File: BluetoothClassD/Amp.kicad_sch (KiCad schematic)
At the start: 31 parts, among them J2 HI OUT, J3 LOW OUT, U4 TPA3110

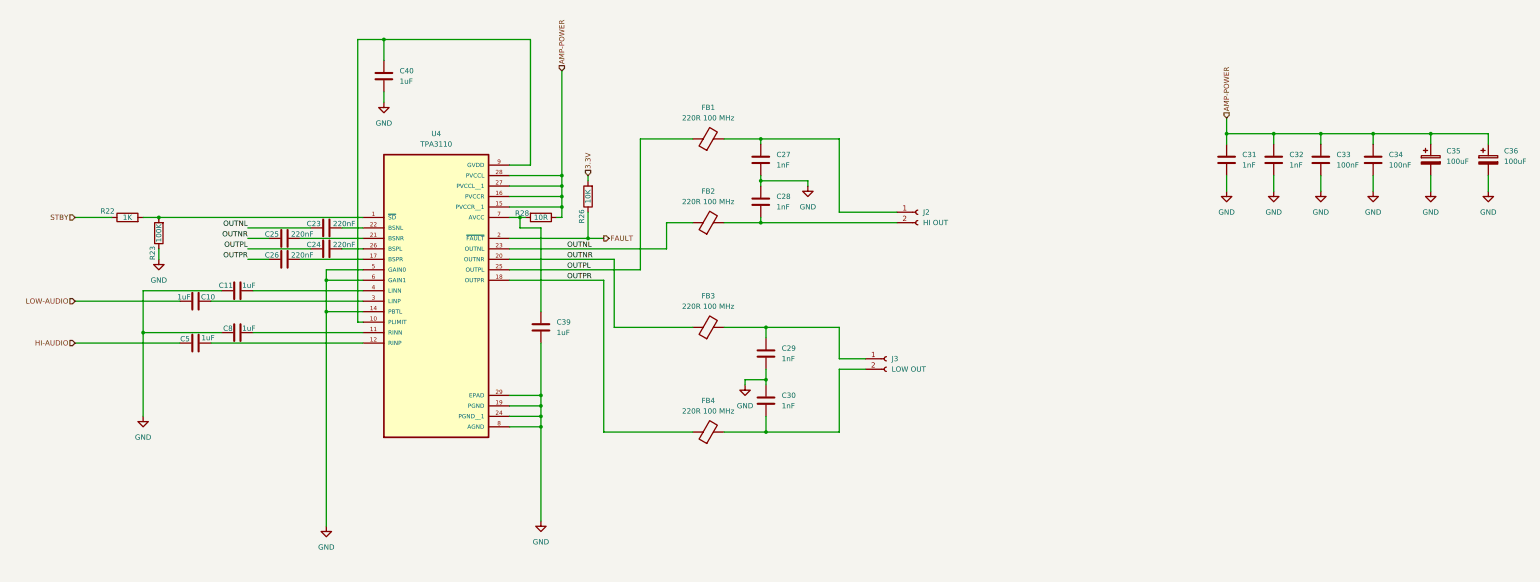
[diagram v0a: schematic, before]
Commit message: work
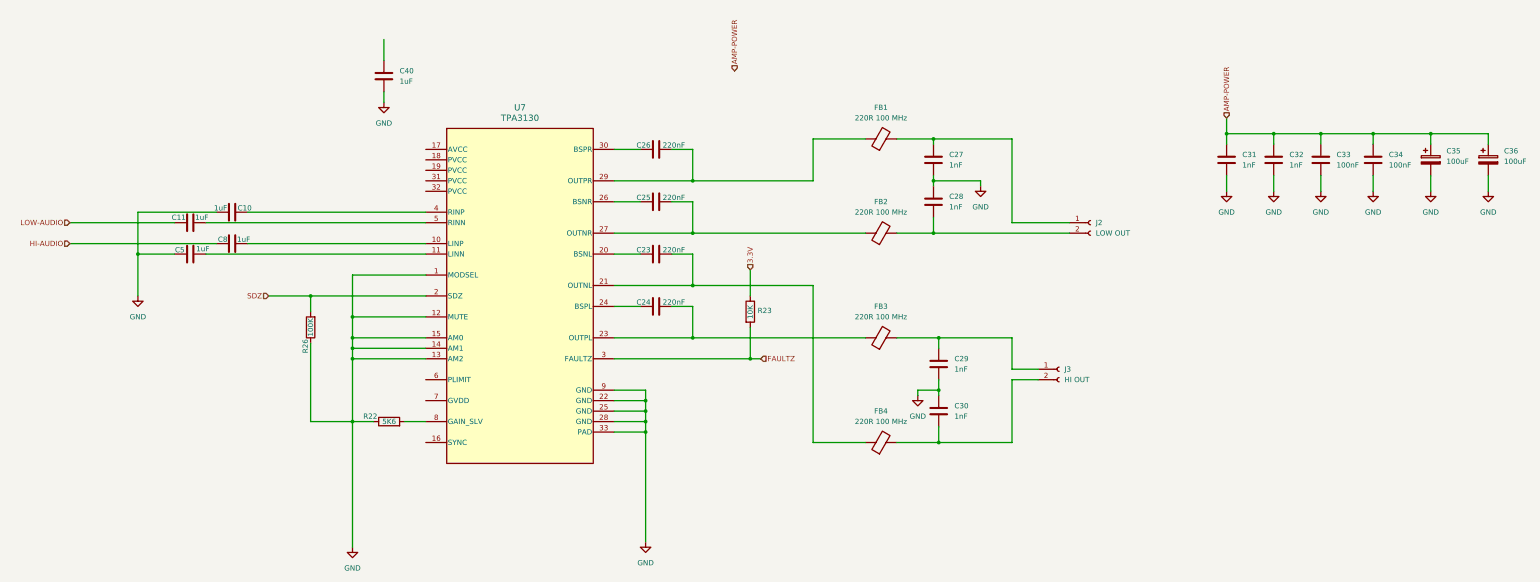
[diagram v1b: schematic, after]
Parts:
- removed C39: 1uF, Capacitor_SMD:C_1206_3216Metric_Pad1.33x1.80mm_HandSolder, symbol Device:C
- removed R28: 10R, Resistor_SMD:R_0805_2012Metric_Pad1.20x1.40mm_HandSolder, symbol Device:R
- removed U4: TPA3110, Custom:TPA3110, symbol Custom:TPA3110D2PWPR
- added U7: TPA3130, Custom:TPA3130D2DAPR, symbol Custom:TPA3130D2DAPR
- J2: value HI OUT -> LOW OUT
- J3: value LOW OUT -> HI OUT
- R22: value 1K -> 5K6
- R23: value 100K -> 10K; footprint Resistor_SMD:R_0805_2012Metric_Pad1.20x1.40mm_HandSolder -> Resistor_SMD:R_0603_1608Metric_Pad0.98x0.95mm_HandSolder
- R26: value 10K -> 100K
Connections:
- net FAULT is gone; now on net GND: R26.1
- net STBY is gone; now on net GND: R22.1
- net 3.3V: now also R23.1; no longer R26.2
- net GND: now also C10.1, C5.1, U7.1 (MODSEL), U7.12 (MUTE), U7.13 (AM2), U7.14 (AM1), U7.15 (AM0), U7.22 (GND), U7.25 (GND), U7.28 (GND), U7.33 (PAD), U7.9 (GND); no longer C11.1, C8.1, R23.1
- net HI-AUDIO: now also C8.1; no longer C5.1
- net LOW-AUDIO: now also C11.1; no longer C10.1
- net at R22.2: now also U7.8 (GAIN_SLV); no longer R23.2
- net at C11.2: now also U7.5 (RINN)
- net at C10.2: now also U7.4 (RINP)
- net at C8.2: now also U7.10 (LINP)
- net at C26.2: now also FB1.1, U7.29 (OUTPR)
- net at C5.2: now also U7.11 (LINN)
- net at C25.2: now also FB2.1, U7.27 (OUTNR)
- net at C23.2: now also FB4.1, U7.21 (OUTNL)
- net at C24.2: now also FB3.1, U7.23 (OUTPL)
- net OUTNL: no longer names the net of C23.1
- net OUTNL: now also U7.20 (BSNL); no longer FB2.1
- net OUTNR: no longer names the net of C25.1
- net OUTNR: now also U7.26 (BSNR); no longer FB3.1
- net OUTPL: no longer names the net of C24.1
- net OUTPL: now also U7.24 (BSPL); no longer FB1.1
- net OUTPR: no longer names the net of C26.1
- net OUTPR: now also U7.30 (BSPR); no longer FB4.1
- new net FAULTZ: R23.2, U7.3 (FAULTZ)
- new net SDZ: R26.2, U7.2 (SDZ)
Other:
- moved on the sheet: C10, C11, C23, C24, C25, C26, C27, C28, C29, C30, C5, C8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
